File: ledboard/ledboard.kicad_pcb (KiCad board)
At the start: 2 copper layers, 100 x 80 mm, 88 parts, among them J1 Barrel_Jack_Switch, J2 Conn_02x20_Odd_Even, J3 Conn_01x02, U1 TPS54332DDA, U2 TPS7A5301BRPSR, U3 TPS2121, U4 TBD62083AFG, U5 TBD62783AFG, U6 TBD62083AFG, U7 TBD62083AFG, U8 TBD62783AFG

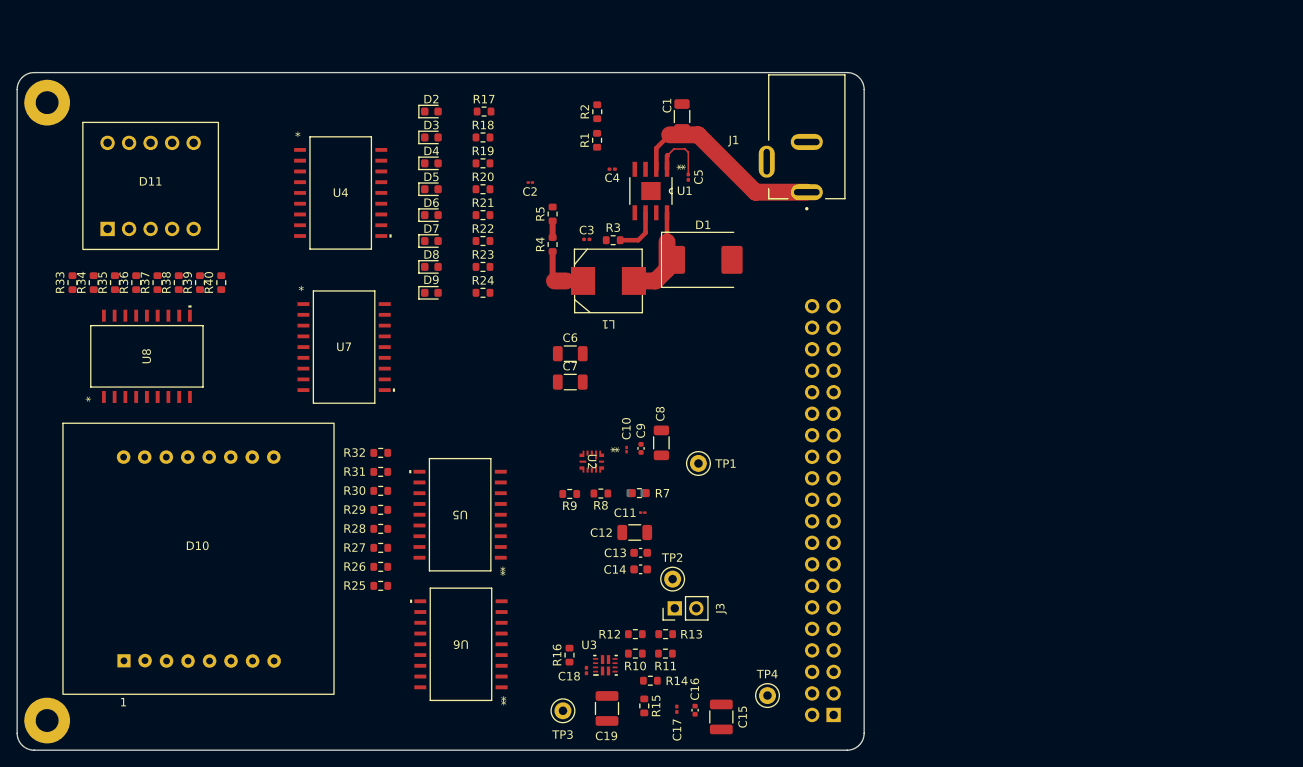
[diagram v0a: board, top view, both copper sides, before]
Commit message: PCBデザイン. 未結線がなくなったところまで.
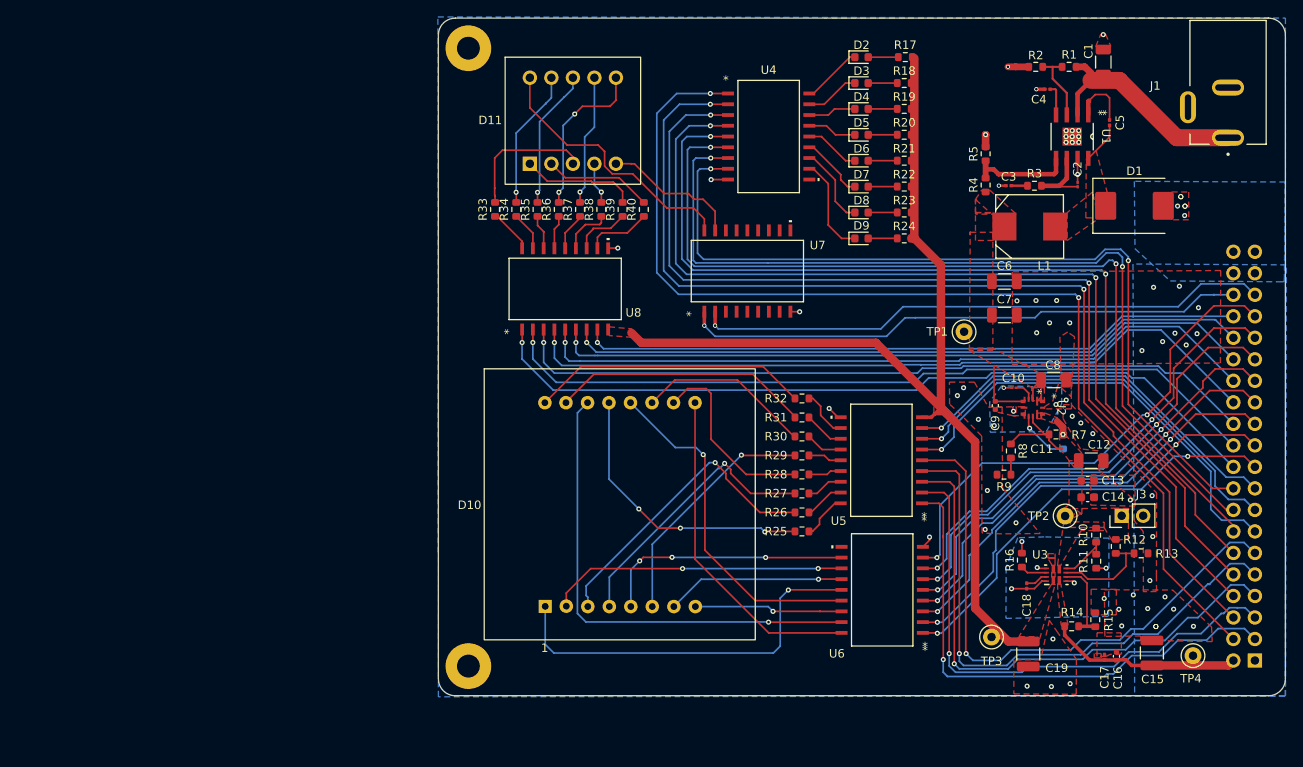
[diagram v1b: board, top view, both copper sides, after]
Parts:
- moved C2 64.6 mm to (166.2, 73.2), turned to 90 degrees
- moved R12 57.7 mm to (170.7, 115.9), turned to -90 degrees
- moved R13 56.9 mm to (173.7, 116.8)
- moved R1 56.4 mm to (165.2, 59.3), turned to 180 degrees
- moved R10 56.2 mm to (168.3, 114.6), turned to -90 degrees
- moved R16 54.6 mm to (159.6, 117.6)
- moved C12 54.6 mm to (167.8, 105.8), turned to 0 degrees
- moved U3 54.3 mm to (163.6, 119.3)
- moved R15 54.2 mm to (168.2, 124.6), turned to 90 degrees
- moved J3 53.9 mm to (171.4, 112.3)
- moved C13 53.5 mm to (167.3, 108.2), turned to 0 degrees
- moved C14 53.5 mm to (167.3, 110.1), turned to 0 degrees
- moved C18 52.9 mm to (160.2, 120.6)
- moved U2 52.5 mm to (160.9, 99.6)
- moved C4 52.2 mm to (162.6, 62.0)
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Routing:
- net /LED_and_Conn/IO1_P: track 0.00 -> 127.1 mm, vias 0 -> 2
- net /LED_and_Conn/IO2_P: track 0.00 -> 122.8 mm, vias 0 -> 2
- net /LED_and_Conn/+5V_VCC: track 0.00 -> 122.2 mm
- net /LED_and_Conn/IO3_P: track 0.00 -> 118.0 mm, vias 0 -> 2
- net /LED_and_Conn/IO4_P: track 0.00 -> 113.6 mm, vias 0 -> 2
- net /LED_and_Conn/IO5_P: track 0.00 -> 109.5 mm, vias 0 -> 2
- net /LED_and_Conn/IO6_P: track 0.00 -> 106.6 mm, vias 0 -> 2
- net /LED_and_Conn/IO7_P: track 0.00 -> 103.3 mm, vias 0 -> 2
- net /LED_and_Conn/IO8_P: track 0.00 -> 99.4 mm, vias 0 -> 2
- net /LED_and_Conn/IO9_P: track 0.00 -> 94.5 mm, vias 0 -> 1
- net /LED_and_Conn/IO10_P: track 0.00 -> 91.7 mm, vias 0 -> 1
- net /LED_and_Conn/IO12_P: track 0.00 -> 89.2 mm, vias 0 -> 1
- net /LED_and_Conn/IO11_P: track 0.00 -> 89.1 mm, vias 0 -> 1
- net /LED_and_Conn/IO13_P: track 0.00 -> 86.8 mm, vias 0 -> 1
- net /LED_and_Conn/IO14_P: track 0.00 -> 83.9 mm, vias 0 -> 1
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- added copper zone on F.Cu, net /+5V
- added copper zone on F.Cu, net /+5V_LOCAL
- added copper zone on F.Cu, net /LED_and_Conn/+5V_VCC
- added copper zone on B.Cu, net GND
- added copper zone on F.Cu, net GND
- added copper zone on F.Cu, net Net-(D1-K)
- added copper zone on F.Cu, net Net-(U2-BIAS)
